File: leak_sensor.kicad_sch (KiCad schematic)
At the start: 3 parts, among them Q4 TP2104N3-G

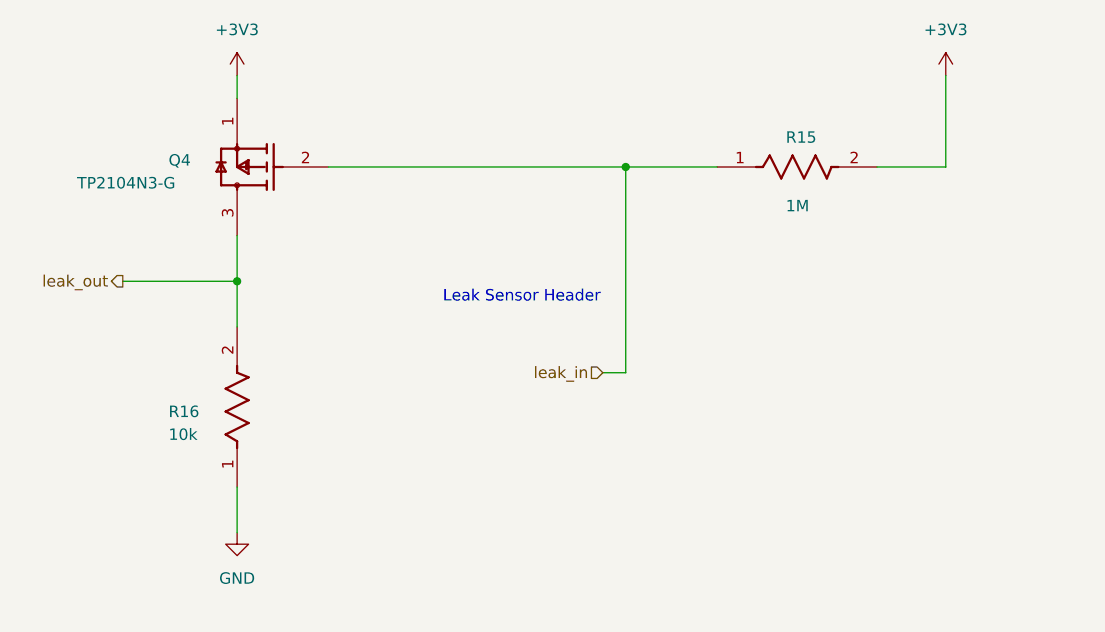
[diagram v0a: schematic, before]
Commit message: Fix a variety of small issues
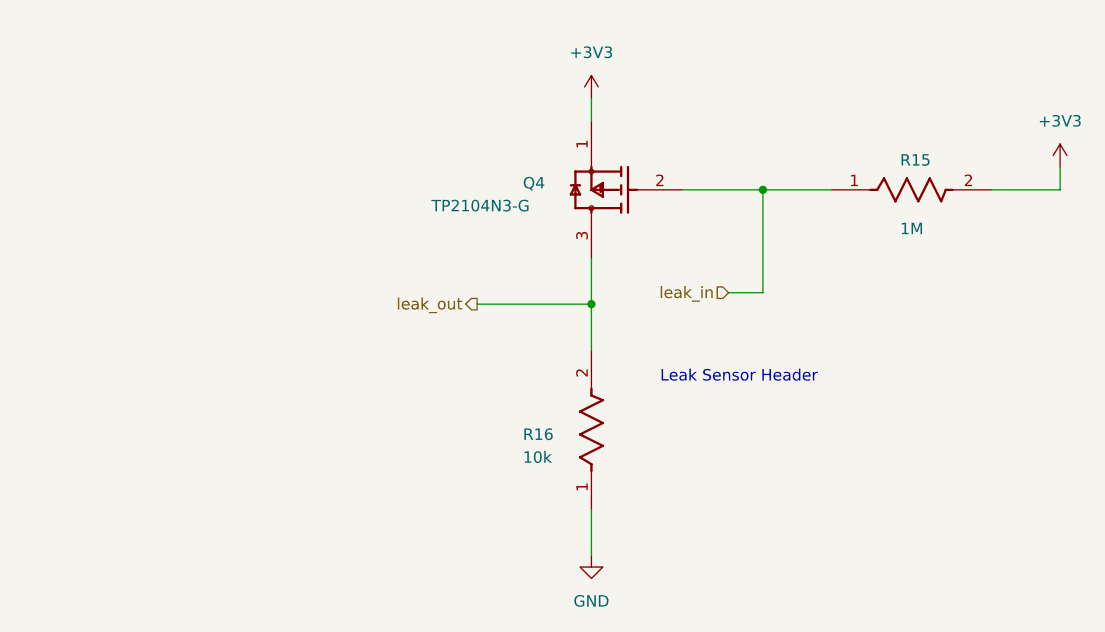
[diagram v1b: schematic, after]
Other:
- moved on the sheet: Q4, R15, R16
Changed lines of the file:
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@@
 (kicad_sch (version 20230121) (generator eeschema)
   (paper "A")
-  (junction (at 81.28 101.6) (diameter 0) (color 0 0 0 0)
+  (junction (at 120.65 104.14) (diameter 0) (color 0 0 0 0)
   )
-  (junction (at 124.46 88.9) (diameter 0) (color 0 0 0 0)
+  (junction (at 139.7 91.44) (diameter 0) (color 0 0 0 0)
   )
-  (wire (pts (xy 124.46 88.9) (xy 124.46 111.76))
+  (wire (pts (xy 139.7 91.44) (xy 139.7 102.87))
     (stroke (width 0.254) (type default))
   )
-  (wire (pts (xy 81.28 129.54) (xy 81.28 124.46))
+  (wire (pts (xy 139.7 102.87) (xy 135.89 102.87))
     (stroke (width 0.254) (type default))
   )
-  (wire (pts (xy 160.02 88.9) (xy 152.4 88.9))
+  (wire (pts (xy 120.65 132.08) (xy 120.65 127))
     (stroke (width 0.254) (type default))
   )
-  (wire (pts (xy 121.92 111.76) (xy 124.46 111.76))
+  (wire (pts (xy 172.72 91.44) (xy 165.1 91.44))
     (stroke (width 0.254) (type default))
   )
-  (wire (pts (xy 160.02 78.74) (xy 160.02 88.9))
+  (wire (pts (xy 172.72 88.9) (xy 172.72 91.44))
     (stroke (width 0.254) (type default))
   )
-  (wire (pts (xy 134.62 88.9) (xy 124.46 88.9))
+  (wire (pts (xy 107.95 104.14) (xy 120.65 104.14))
     (stroke (width 0.254) (type default))
   )
-  (wire (pts (xy 68.58 101.6) (xy 81.28 101.6))
+  (wire (pts (xy 120.65 104.14) (xy 120.65 99.06))
     (stroke (width 0.254) (type default))
   )
-  (wire (pts (xy 124.46 88.9) (xy 91.44 88.9))
+  (wire (pts (xy 120.65 81.28) (xy 120.65 83.82))
     (stroke (width 0.254) (type default))
   )
-  (wire (pts (xy 81.28 101.6) (xy 81.28 96.52))
+  (wire (pts (xy 120.65 104.14) (xy 120.65 109.22))
     (stroke (width 0.254) (type default))
   )
-  (wire (pts (xy 81.28 78.74) (xy 81.28 81.28))
+  (wire (pts (xy 139.7 91.44) (xy 147.32 91.44))
     (stroke (width 0.254) (type default))
   )
-  (wire (pts (xy 81.28 101.6) (xy 81.28 106.68))
+  (wire (pts (xy 130.81 91.44) (xy 139.7 91.44))
     (stroke (width 0.254) (type default))
   )
-  (text "Leak Sensor Header" (at 104.14 104.14 0)
+  (text "Leak Sensor Header" (at 128.27 113.03 0)
     (effects (font (size 1.27 1.27)) (justify left bottom))
   )
-  (hierarchical_label "leak_out" (shape output) (at 68.58 101.6 180) (fields_autoplaced)
+  (hierarchical_label "leak_out" (shape output) (at 107.95 104.14 180) (fields_autoplaced)
     (effects (font (size 1.27 1.27)) (justify right))
   )
-  (hierarchical_label "leak_in" (shape input) (at 121.92 111.76 180) (fields_autoplaced)
+  (hierarchical_label "leak_in" (shape input) (at 135.89 102.87 180) (fields_autoplaced)
     (effects (font (size 1.27 1.27)) (justify right))
   )
-  (symbol (lib_id "MEB-altium-import:leak_sensor_1_1029c3af85768c4190bb7ad29bc67b5") (at 81.28 124.46 0) (unit 1)
+  (symbol (lib_id "MEB-altium-import:leak_sensor_1_1029c3af85768c4190bb7ad29bc67b5") (at 120.65 127 0) (unit 1)
     (in_bom yes) (on_board yes) (dnp no)
-    (property "Reference" "R16" (at 73.66 116.84 0)
+    (property "Reference" "R16" (at 113.03 119.38 0)
       (effects (font (size 1.27 1.27)) (justify left bottom))
     )
-    (property "Value" "10k" (at 73.66 119.38 0)
+    (property "Value" "10k" (at 113.03 121.92 0)
       (effects (font (size 1.27 1.27)) (justify left bottom))
     )
-    (property "Footprint" "Resistor_SMD:R_0805_2012Metric_Pad1.20x1.40mm_HandSolder" (at 81.28 124.46 0)
+    (property "Footprint" "Resistor_SMD:R_0805_2012Metric_Pad1.20x1.40mm_HandSolder" (at 120.65 127 0)
       (effects (font (size 1.27 1.27)) hide)
     )
-    (property "Datasheet" "" (at 81.28 124.46 0)
+    (property "Datasheet" "" (at 120.65 127 0)
       (effects (font (size 1.27 1.27)) hide)
     )
-    (property "Part Number" "RNCP0805FTD10K0" (at 81.28 124.46 0)
+    (property "Part Number" "RNCP0805FTD10K0" (at 120.65 127 0)
       (effects (font (size 1.27 1.27)) hide)
     )
@@
     )
   )
-  (symbol (lib_id "power:GND") (at 81.28 129.54 0) (unit 1)
+  (symbol (lib_id "power:GND") (at 120.65 132.08 0) (unit 1)
     (in_bom yes) (on_board yes) (dnp no) (fields_autoplaced)
-    (property "Reference" "#PWR030" (at 81.28 135.89 0)
+    (property "Reference" "#PWR027" (at 120.65 138.43 0)
       (effects (font (size 1.27 1.27)) hide)
     )
-    (property "Value" "GND" (at 81.28 134.62 0)
+    (property "Value" "GND" (at 120.65 137.16 0)
       (effects (font (size 1.27 1.27)))
     )
-    (property "Footprint" "" (at 81.28 129.54 0)
+    (property "Footprint" "" (at 120.65 132.08 0)
       (effects (font (size 1.27 1.27)) hide)
     )
-    (property "Datasheet" "" (at 81.28 129.54 0)
+    (property "Datasheet" "" (at 120.65 132.08 0)
       (effects (font (size 1.27 1.27)) hide)
     )
@@
     (instances
       (project "MEB"
-        (path "/228e4997-23c1-4c21-939b-583cad26a5e3/3aab6a70-cc66-4393-a750-92acad576aaa"
-          (reference "#PWR030") (unit 1)
-        )
         (path "/228e4997-23c1-4c21-939b-583cad26a5e3/0dfd1422-c5d3-49c9-a73a-0802f4b457f4"
           (reference "#PWR027") (unit 1)
@@
     )
   )
-  (symbol (lib_id "MEB-altium-import:leak_sensor_2_9a74f65b4248df6e06e844fd3676475") (at 91.44 88.9 0) (unit 1)
+  (symbol (lib_id "MEB-altium-import:leak_sensor_2_9a74f65b4248df6e06e844fd3676475") (at 130.81 91.44 0) (unit 1)
     (in_bom yes) (on_board yes) (dnp no)
-    (property "Reference" "Q4" (at 73.66 88.9 0)
+    (property "Reference" "Q4" (at 113.03 91.44 0)
       (effects (font (size 1.27 1.27)) (justify left bottom))
     )
-    (property "Value" "TP2104N3-G" (at 63.5 91.44 0)
+    (property "Value" "TP2104N3-G" (at 102.87 93.98 0)
       (effects (font (size 1.27 1.27)) (justify left bottom))
     )
-    (property "Footprint" "AltiumImport:FP-TP2104N3-G-MFG" (at 91.44 88.9 0)
+    (property "Footprint" "AltiumImport:FP-TP2104N3-G-MFG" (at 130.81 91.44 0)
       (effects (font (size 1.27 1.27)) hide)
     )
-    (property "Datasheet" "" (at 91.44 88.9 0)
+    (property "Datasheet" "" (at 130.81 91.44 0)
       (effects (font (size 1.27 1.27)) hide)
     )
-    (property "Part Number" "TP2104N3-G" (at 91.44 88.9 0)
+    (property "Part Number" "TP2104N3-G" (at 130.81 91.44 0)
       (effects (font (size 1.27 1.27)) hide)
     )
@@
     )
   )
-  (symbol (lib_id "power:+3V3") (at 81.28 78.74 0) (unit 1)
+  (symbol (lib_id "power:+3V3") (at 120.65 81.28 0) (unit 1)
     (in_bom yes) (on_board yes) (dnp no) (fields_autoplaced)
-    (property "Reference" "#PWR036" (at 81.28 82.55 0)
+    (property "Reference" "#PWR037" (at 120.65 85.09 0)
       (effects (font (size 1.27 1.27)) hide)
     )
-    (property "Value" "+3V3" (at 81.28 73.66 0)
+    (property "Value" "+3V3" (at 120.65 76.2 0)
       (effects (font (size 1.27 1.27)))
     )
-    (property "Footprint" "" (at 81.28 78.74 0)
+    (property "Footprint" "" (at 120.65 81.28 0)
       (effects (font (size 1.27 1.27)) hide)
     )
-    (property "Datasheet" "" (at 81.28 78.74 0)
+    (property "Datasheet" "" (at 120.65 81.28 0)
       (effects (font (size 1.27 1.27)) hide)
     )
@@
     (instances
       (project "MEB"
-        (path "/228e4997-23c1-4c21-939b-583cad26a5e3"
-          (reference "#PWR036") (unit 1)
-        )
         (path "/228e4997-23c1-4c21-939b-583cad26a5e3/0dfd1422-c5d3-49c9-a73a-0802f4b457f4"
           (reference "#PWR037") (unit 1)
@@
     )
   )
-  (symbol (lib_id "power:+3V3") (at 160.02 78.74 0) (unit 1)
+  (symbol (lib_id "power:+3V3") (at 172.72 88.9 0) (unit 1)
     (in_bom yes) (on_board yes) (dnp no) (fields_autoplaced)
-    (property "Reference" "#PWR036" (at 160.02 82.55 0)
+    (property "Reference" "#PWR038" (at 172.72 92.71 0)
       (effects (font (size 1.27 1.27)) hide)
     )
-    (property "Value" "+3V3" (at 160.02 73.66 0)
+    (property "Value" "+3V3" (at 172.72 83.82 0)
       (effects (font (size 1.27 1.27)))
     )
-    (property "Footprint" "" (at 160.02 78.74 0)
+    (property "Footprint" "" (at 172.72 88.9 0)
       (effects (font (size 1.27 1.27)) hide)
     )
-    (property "Datasheet" "" (at 160.02 78.74 0)
+    (property "Datasheet" "" (at 172.72 88.9 0)
       (effects (font (size 1.27 1.27)) hide)
     )
@@
     (instances
       (project "MEB"
-        (path "/228e4997-23c1-4c21-939b-583cad26a5e3"
-          (reference "#PWR036") (unit 1)
-        )
         (path "/228e4997-23c1-4c21-939b-583cad26a5e3/0dfd1422-c5d3-49c9-a73a-0802f4b457f4"
           (reference "#PWR038") (unit 1)
@@
     )
   )
-  (symbol (lib_id "MEB-altium-import:leak_sensor_0_1029c3af85768c4190bb7ad29bc67b5") (at 134.62 88.9 0) (unit 1)
+  (symbol (lib_id "MEB-altium-import:leak_sensor_0_1029c3af85768c4190bb7ad29bc67b5") (at 147.32 91.44 0) (unit 1)
     (in_bom yes) (on_board yes) (dnp no)
-    (property "Reference" "R15" (at 142.24 86.36 0)
+    (property "Reference" "R15" (at 154.94 88.9 0)
       (effects (font (size 1.27 1.27)) (justify left bottom))
     )
-    (property "Value" "1M" (at 142.24 93.98 0)
+    (property "Value" "1M" (at 154.94 96.52 0)
       (effects (font (size 1.27 1.27)) (justify left bottom))
     )
-    (property "Footprint" "Resistor_SMD:R_0805_2012Metric_Pad1.20x1.40mm_HandSolder" (at 134.62 88.9 0)
+    (property "Footprint" "Resistor_SMD:R_0805_2012Metric_Pad1.20x1.40mm_HandSolder" (at 147.32 91.44 0)
       (effects (font (size 1.27 1.27)) hide)
     )
-    (property "Datasheet" "" (at 134.62 88.9 0)
+    (property "Datasheet" "" (at 147.32 91.44 0)
       (effects (font (size 1.27 1.27)) hide)
     )
-    (property "Part Number" "RMCF0805JT1M00" (at 134.62 88.9 0)
+    (property "Part Number" "RMCF0805JT1M00" (at 147.32 91.44 0)
       (effects (font (size 1.27 1.27)) hide)
     )
